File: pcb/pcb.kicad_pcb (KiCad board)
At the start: 2 copper layers, 40.9 x 47.8 mm, 45 parts, among them J1 USB-C, J2 Battery, J3 Soil_Sensor, J4 Pump, J5 Water_Sensor, Q1 AO3401A, Q2 AO3400A, U1 TPS63802DLAR, U2 BQ24075RGTR, U3 ESP-32S DevBoard

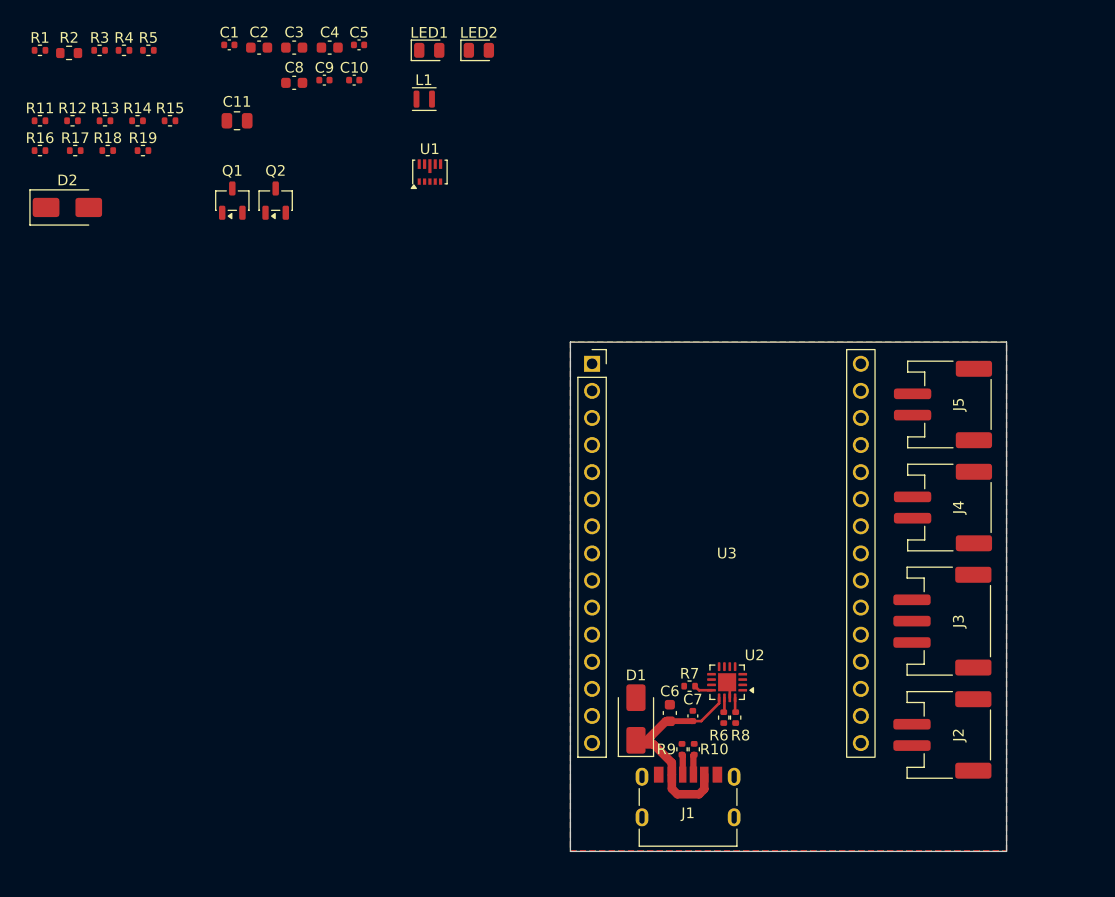
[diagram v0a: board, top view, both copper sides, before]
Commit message: Finished first iteration of the new PCB design
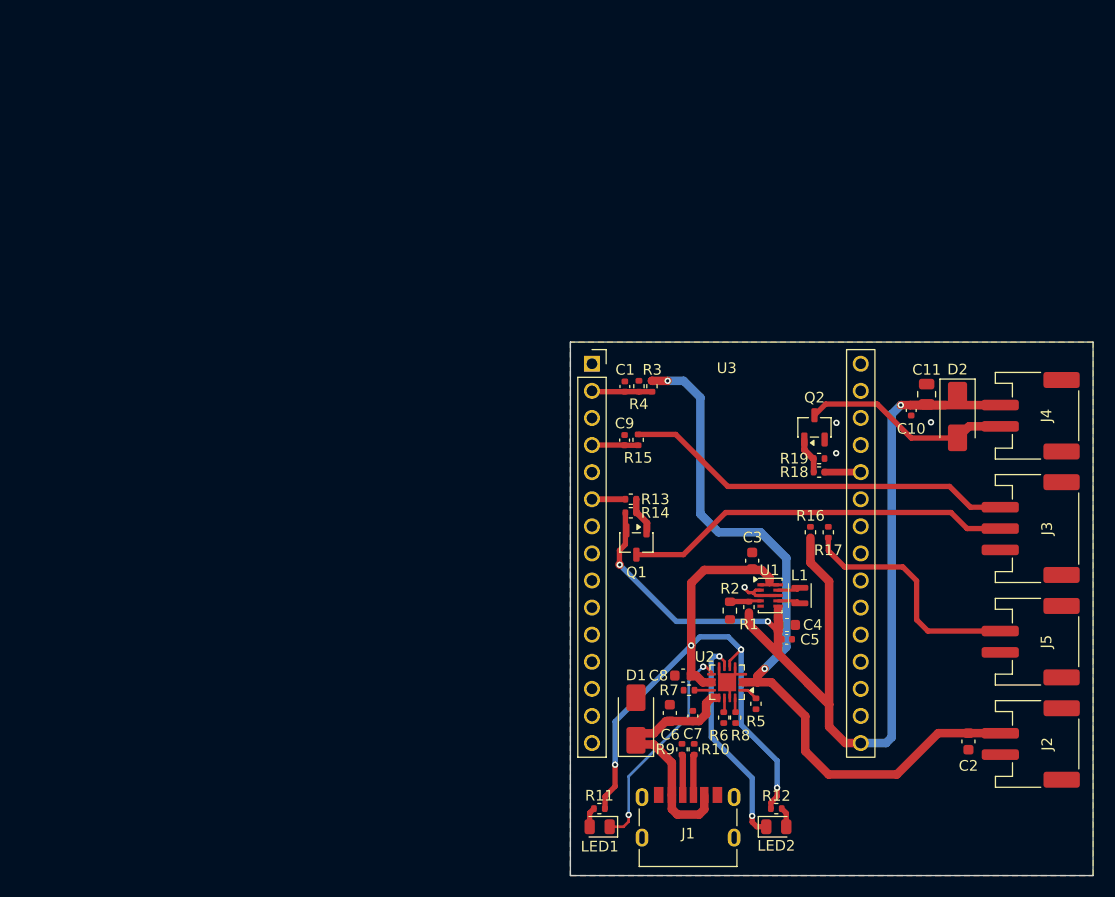
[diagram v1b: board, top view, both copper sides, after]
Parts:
- moved C2 93.0 mm to (139.7, 103.2), turned to -90 degrees
- moved R12 92.3 mm to (121.7, 109.5), turned to 180 degrees
- moved D2 85.7 mm to (138.7, 72.8), turned to -90 degrees
- moved R1 84.5 mm to (119.1, 90.6), turned to -90 degrees
- moved R5 83.7 mm to (119.8, 99.7), turned to 90 degrees
- moved R11 83.1 mm to (105.1, 109.5)
- moved R2 81.1 mm to (117.3, 91.0), turned to 90 degrees
- moved R16 80.6 mm to (124.9, 83.6), turned to -90 degrees
- moved R17 79.2 mm to (126.5, 83.6), turned to 90 degrees
- moved LED2 78.0 mm to (121.7, 111.2)
- moved LED1 74.5 mm to (105.1, 111.2), turned to 180 degrees
- moved R18 73.2 mm to (125.7, 78.0), turned to 180 degrees
- moved R19 69.7 mm to (125.7, 76.7), turned to 180 degrees
- moved C11 69.6 mm to (135.8, 70.7), turned to 90 degrees
- moved C4 69.1 mm to (122.7, 92.3), turned to 180 degrees
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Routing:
- net +3.3V: track 0.00 -> 111.6 mm, vias 0 -> 3
- net Net-(C2-Pad1): track 0.00 -> 71.7 mm, vias 0 -> 2
- net VIMM: track 0.00 -> 63.8 mm, vias 0 -> 4
- net Net-(J3-Pad3): track 0.00 -> 36.8 mm
- net Net-(Q1-D): track 0.00 -> 36.4 mm
- net Net-(J5-Pad2): track 0.00 -> 22.6 mm
- net Net-(U2-#CHG): track 0.00 -> 20.6 mm, vias 0 -> 2
- net Net-(U2-#PGOOD): track 0.00 -> 20.4 mm, vias 0 -> 2
- net Net-(Q2-D): track 0.00 -> 19.6 mm
- net GND: track 1.57 -> 9.97 mm, vias 0 -> 4
- net BAT_SENSE: track 0.00 -> 5.65 mm
- net SOIL_OUT: track 0.00 -> 4.34 mm
- net Net-(Q2-G): track 0.00 -> 3.47 mm
- net Net-(Q1-G): track 0.00 -> 3.39 mm
- net ~{SOIL_ON}: track 0.00 -> 3.13 mm
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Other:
- board size 40.9 x 47.8 mm -> 49 x 50 mm
